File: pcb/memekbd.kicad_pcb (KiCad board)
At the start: 2 copper layers, 134.1 x 130.9 mm, 209 parts, among them J1 AudioJack4, J2 AudioJack4, SW1 SW_Push, SW10 SW_Push, SW11 SW_Push, SW12 SW_Push, SW13 SW_Push, SW14 SW_Push, SW15 SW_Push, SW16 SW_Push, SW17 SW_Push, SW18 SW_Push, SW19 SW_Push, SW2 SW_Push, SW20 SW_Push, SW21 SW_Push, SW22 SW_Push, SW23 SW_Push, SW24 SW_Push, SW25 SW_Push, SW26 SW_Push, SW27 SW_Push, SW28 SW_Push, SW29 SW_Push, SW3 SW_Push, SW30 SW_Push, SW31 SW_Push, SW32 SW_Push, SW33 SW_Push, SW34 SW_Push, SW35 SW_Push, SW36 SW_Push, SW37 SW_Push, SW38 SW_Push, SW39 SW_Push, SW4 SW_Push, SW40 SW_Push, SW41 SW_Push, SW42 SW_Push, SW43 SW_Push, SW44 SW_Push, SW45 SW_Push, SW46 SW_Push, SW47 SW_Push, SW48 SW_Push, SW5 SW_Push, SW6 SW_Push, SW7 SW_Push, SW8 SW_Push, SW9 SW_Push, U1 ProMicro, U2 ProMicro

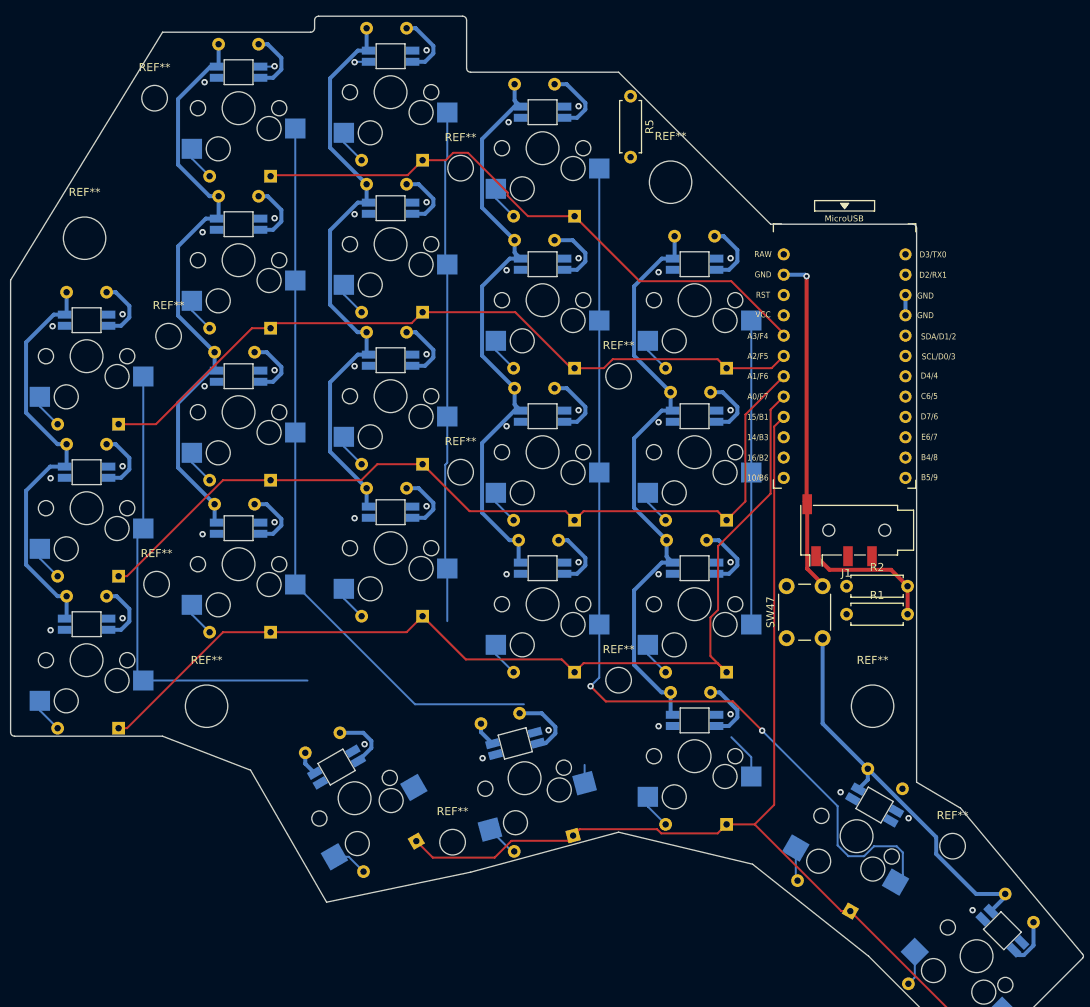
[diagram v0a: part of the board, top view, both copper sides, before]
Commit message: Routing progress
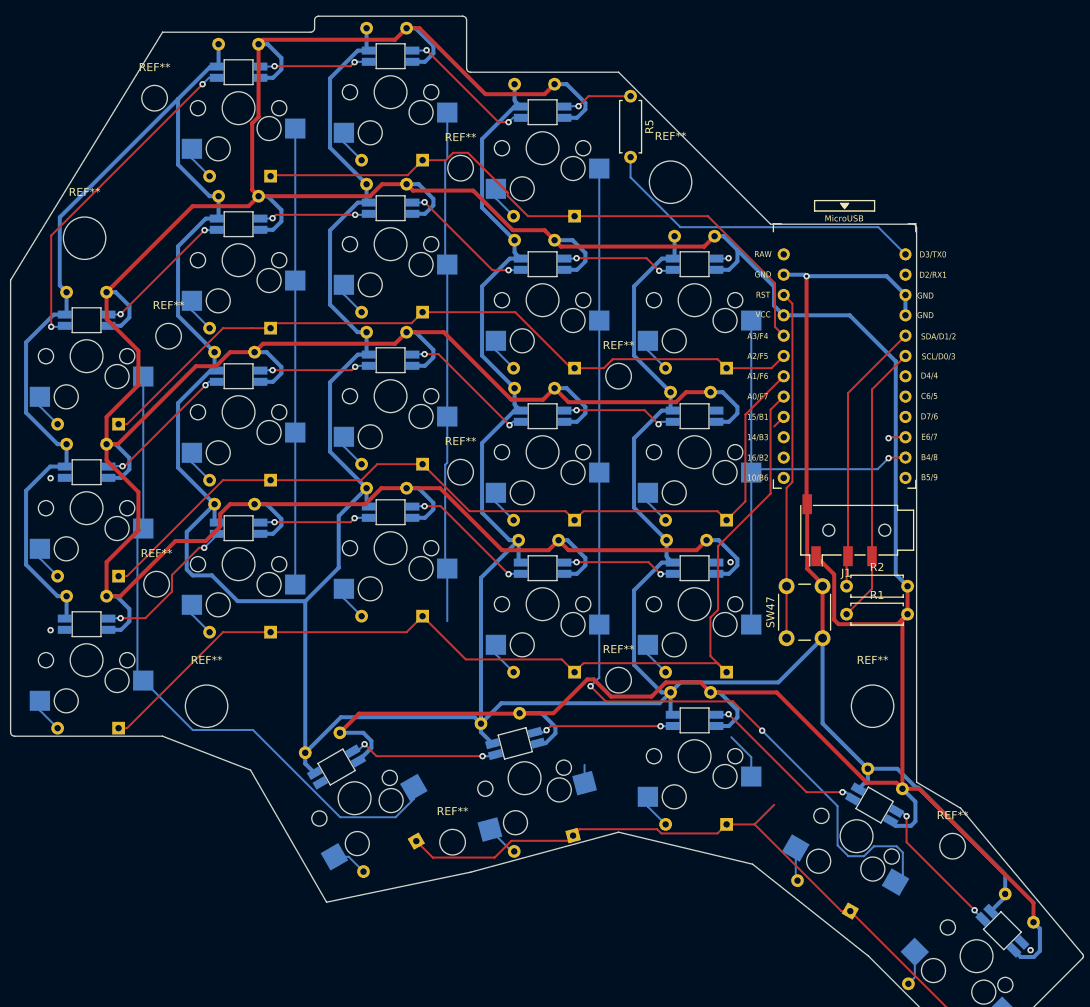
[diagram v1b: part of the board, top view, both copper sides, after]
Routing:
- net +5V: track 194.4 -> 758.4 mm
- net GND: track 452.3 -> 661.4 mm
- net /lrow4: track 133.9 -> 86.6 mm
- net /lRST: track 0.00 -> 43.6 mm
- net Net-(LED1-Pad4): track 0.00 -> 42.0 mm, vias 0 -> 2
- net /lLED: track 0.00 -> 40.9 mm
- net /lSCL: track 0.00 -> 35.3 mm
- net /lcol1: track 94.1 -> 59.3 mm
- net /lSDA: track 0.00 -> 34.4 mm
- net /lcol0: track 59.2 -> 82.0 mm
- net Net-(LED14-Pad2): track 0.00 -> 21.4 mm, vias 0 -> 2
- net /lcol4: track 38.0 -> 58.1 mm, vias 0 -> 1
- net Net-(LED3-Pad2): track 0.00 -> 19.2 mm, vias 0 -> 2
- net Net-(LED4-Pad2): track 0.00 -> 18.9 mm, vias 0 -> 2
- net Net-(LED19-Pad2): track 0.00 -> 18.3 mm, vias 0 -> 2
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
